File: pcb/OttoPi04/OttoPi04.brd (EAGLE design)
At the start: 48.3 x 63.5 mm, 26 parts

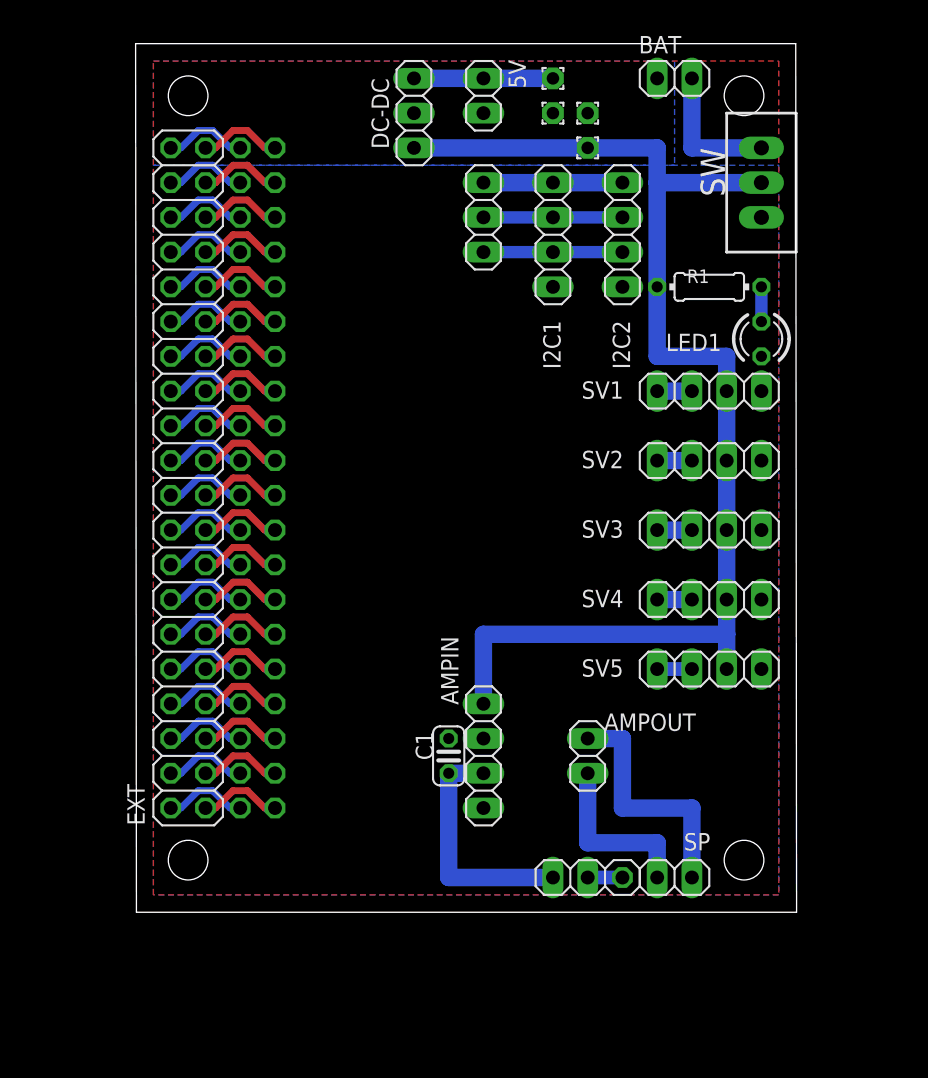
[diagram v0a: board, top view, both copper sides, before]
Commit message: pcb
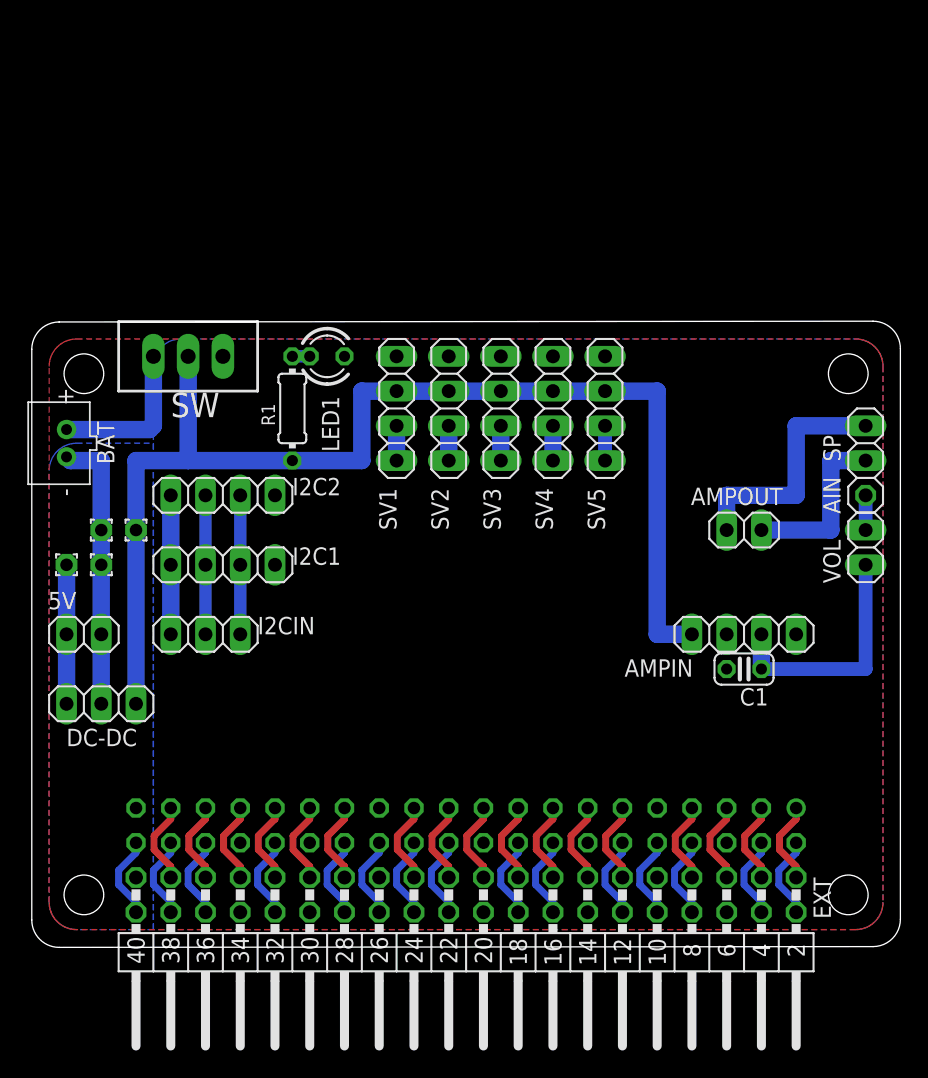
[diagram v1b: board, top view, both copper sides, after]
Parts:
- BAT: device pinhead:1X02 -> adafruit:JST-PH-2-THM
- EXT: device pinhead:2X20 -> con-lstb:MA20-2W
- RPI: device pinhead:2X20 -> con-lsta:FE20-2
- moved BAT 51.8 mm to (2.54, 36.8), turned to 90 degrees
- moved 5V_A 50.3 mm to (2.54, 27.9), turned to 90 degrees
- moved 5V 49.0 mm to (3.81, 22.9), turned to 0 degrees
- moved DC-DC 48.9 mm to (5.08, 17.8), turned to 180 degrees
- moved GND_B 46.8 mm to (5.08, 30.5), turned to 90 degrees
- moved GND_A 46.7 mm to (5.08, 27.9), turned to 90 degrees
- moved SW 43.8 mm to (11.4, 43.2), turned to 0 degrees
- moved BAT_B 43.3 mm to (7.62, 30.5), turned to 90 degrees
- moved I2CIN 36.6 mm to (12.7, 22.9), turned to 0 degrees
- moved EXT 36.6 mm to (31.8, 3.81), turned to 180 degrees
- moved I2C2 34.9 mm to (14.0, 33.0), turned to 0 degrees
- moved SP 34.7 mm to (61.0, 36.8), turned to 270 degrees
- moved I2C1 34.1 mm to (14.0, 27.9), turned to 0 degrees
- moved AIN 33.1 mm to (61.0, 33.0), turned to 270 degrees
- moved VOL 32.4 mm to (61.0, 29.2), turned to 270 degrees
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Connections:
- net 3V3 renamed +3V3
- net 5V renamed +5V
- removed net 3V: EXT.1, RPI.2
- removed net 4V: AMPIN.4, BAT_B.1, DC-DC.1, R1.2, SV1.2, SV2.2, SV3.2, SV4.2, SV5.2, SW.2
- removed net 5V1: EXT.2, RPI.1
- removed net 5V2: EXT.4, RPI.3
- removed net N$1: EXT.28, RPI.27
- removed net N$10: EXT.7, RPI.8
- removed net N$12: EXT.11, RPI.12
- removed net N$13: EXT.13, RPI.14
- removed net N$14: EXT.15, RPI.16
- removed net N$17: EXT.19, RPI.20
- removed net N$18: EXT.21, RPI.22
- removed net N$19: EXT.23, RPI.24
- removed net N$2: EXT.17, RPI.18
- removed net N$21: EXT.27, RPI.28
- removed net N$22: EXT.29, RPI.30
- removed net N$23: EXT.31, RPI.32
- removed net N$24: EXT.33, RPI.34
- removed net N$25: EXT.35, RPI.36
- removed net N$26: EXT.37, RPI.38
- removed net N$28: EXT.12, RPI.11
- removed net N$30: EXT.16, RPI.15
- removed net N$31: EXT.40, RPI.39
- removed net N$32: EXT.38, RPI.37
- removed net N$35: EXT.32, RPI.31
- removed net N$38: EXT.26, RPI.25
- removed net N$39: EXT.24, RPI.23
- removed net N$4: EXT.3, RPI.4
- removed net N$41: EXT.18, RPI.17
- removed net N$43: EXT.10, RPI.9
- removed net N$5: EXT.5, RPI.6
- removed net N$6: EXT.22, RPI.21
- removed net N$7: EXT.36, RPI.35
- removed net N$9: EXT.8, RPI.7
- new net +3V3-S1: EXT.1, RPI.1
- new net +3V3-S2: EXT.17, RPI.17
- new net +4V_S: BAT.1, SW.1
- new net +5V-S1: EXT.2, RPI.2
- new net +5V-S2: EXT.4, RPI.4
- new net GPIO0: EXT.27, RPI.27
- new net GPIO1: EXT.28, RPI.28
- new net GPIO10: EXT.19, RPI.19
- new net GPIO11: EXT.23, RPI.23
- new net GPIO12: EXT.32, RPI.32
- new net GPIO13: EXT.33, RPI.33
- new net GPIO14: EXT.8, RPI.8
- new net GPIO15: EXT.10, RPI.10
- new net GPIO16: EXT.36, RPI.36
- new net GPIO17: EXT.11, RPI.11
- new net GPIO18: EXT.12, RPI.12
- new net GPIO19: EXT.35, RPI.35
- new net GPIO20: EXT.38, RPI.38
- new net GPIO21: EXT.40, RPI.40
- new net GPIO22: EXT.15, RPI.15
- new net GPIO23: EXT.16, RPI.16
- new net GPIO24: EXT.18, RPI.18
- new net GPIO25: EXT.22, RPI.22
- new net GPIO26: EXT.37, RPI.37
- new net GPIO27: EXT.13, RPI.13
- new net GPIO4: EXT.7, RPI.7
- new net GPIO5: EXT.29, RPI.29
- new net GPIO6: EXT.31, RPI.31
- new net GPIO7: EXT.26, RPI.26
- new net GPIO8: EXT.24, RPI.24
- new net GPIO9: EXT.21, RPI.21
- new net SCL-S: EXT.5, RPI.5
- new net SDA-S: EXT.3, RPI.3
- net BAT+: now also AMPIN.4, BAT_B.1, DC-DC.1, R1.2, SV1.2, SV2.2, SV3.2, SV4.2, SV5.2, SW.2; no longer BAT.2, SW.1
- net GND: now also AMPIN.1, BAT.2, RPI.14, RPI.20, RPI.25, RPI.30, RPI.34, RPI.39, RPI.6, RPI.9; no longer BAT.1, RPI.10, RPI.13, RPI.19, RPI.26, RPI.29, RPI.33, RPI.40, RPI.5
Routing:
- net 4V: track 91.4 -> 0.00 mm
- net BAT+: track 10.2 -> 90.2 mm
- net GND: track 49.1 -> 20.4 mm
- net +4V_S: track 0.00 -> 11.5 mm
- net N$24: track 6.13 -> 0.00 mm
- net N$23: track 6.13 -> 0.00 mm
- net N$22: track 6.13 -> 0.00 mm
- net N$21: track 6.13 -> 0.00 mm
- net N$13: track 6.13 -> 0.00 mm
- net GPIO24: track 0.00 -> 6.13 mm
- net GPIO23: track 0.00 -> 6.13 mm
- net GPIO18: track 0.00 -> 6.13 mm
- net +5V-S2: track 0.00 -> 6.13 mm
- net +5V-S1: track 0.00 -> 6.13 mm
- net N$5: track 6.13 -> 0.00 mm
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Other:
- board size 48.3 x 63.5 mm -> 63.5 x 45.8 mm
